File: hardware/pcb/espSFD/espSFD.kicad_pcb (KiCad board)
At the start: 2 copper layers, 68.6 x 34.3 mm, 9 parts, among them J1 Conn_01x06_Socket, J2 Conn_02x10_Odd_Even, Q1 IRLU3110Z, U1 WeMos_D1_mini, U2 TSR_1-2415

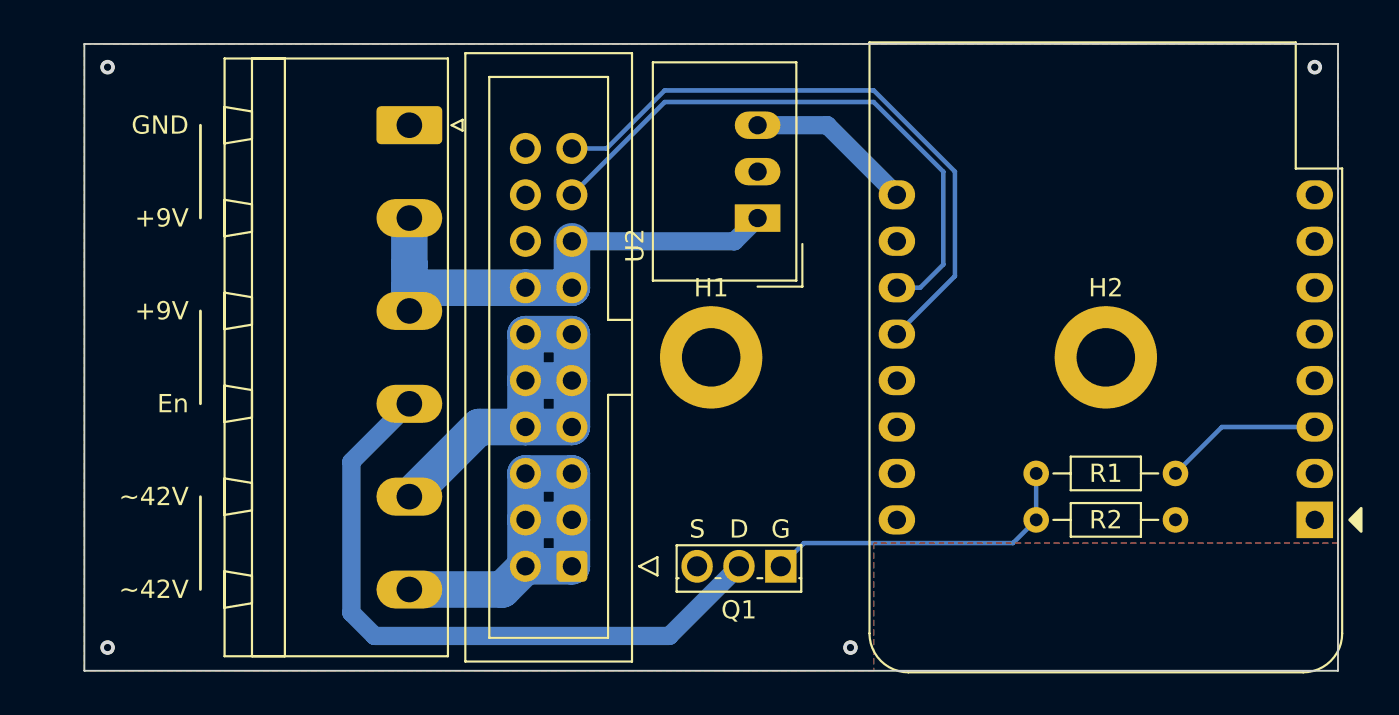
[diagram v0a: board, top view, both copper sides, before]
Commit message: es dghdgfj fcgj
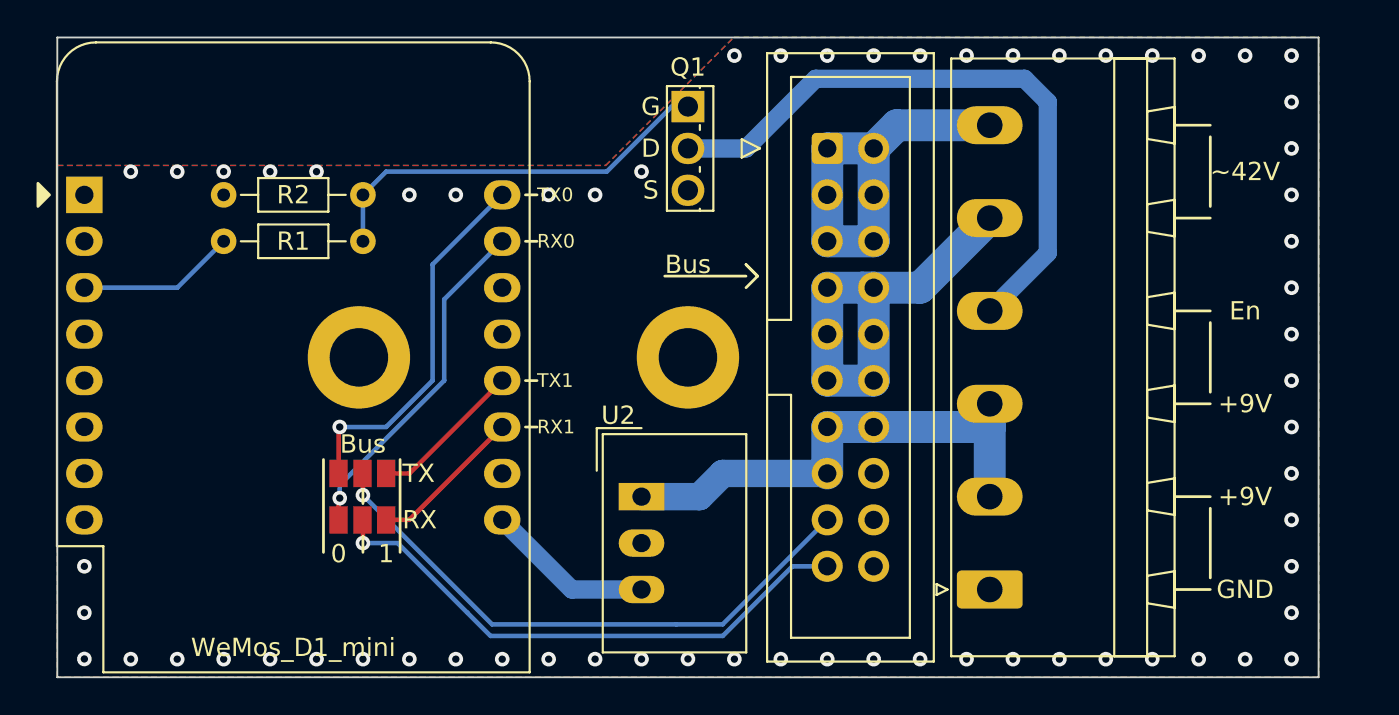
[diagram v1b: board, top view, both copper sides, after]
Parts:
- added JP1: SolderJumper_3_Open, Library:SolderJumper-3_P1.3mm_Open_Pad1.0x1.5mm no silk, F.Cu at (66.0, 102.9)
- added JP2: SolderJumper_3_Open, Library:SolderJumper-3_P1.3mm_Open_Pad1.0x1.5mm no silk, F.Cu at (66.0, 100.3)
- moved U1 69.6 mm to (50.8, 85.1), turned to 0 degrees
- moved R1 53.6 mm to (58.4, 87.6), turned to 0 degrees
- moved R2 40.9 mm to (66.0, 85.1), turned to 180 degrees
- moved H2 40.9 mm to (65.8, 94.0), turned to 180 degrees
- moved J1 40.7 mm to (100.3, 106.7), turned to 90 degrees
- moved J2 26.8 mm to (91.4, 82.5), turned to 0 degrees
- moved Q1 25.7 mm to (83.8, 80.3), turned to -90 degrees
- moved U2 16.5 mm to (81.3, 101.6), turned to -90 degrees
- moved H1 1.27 mm to (83.8, 94.0), turned to 180 degrees
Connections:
- J2 pad 17: RX -> TX
- J2 pad 19: TX -> RX
- U1 pad 11: RX -> RX1
- U1 pad 12: TX -> TX1
- U1 pad 15: unconnected-(U1-RX-Pad15) -> RX0
- U1 pad 16: unconnected-(U1-TX-Pad16) -> TX0
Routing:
- net TX0: track 0.00 -> 20.4 mm, vias 0 -> 1
- net RX0: track 0.00 -> 19.6 mm, vias 0 -> 1
- net TX1: track 0.00 -> 8.45 mm
- net RX1: track 0.00 -> 8.45 mm
- net Net-(Q1-G): track 17.6 -> 22.3 mm
- net Motor N: track 24.7 -> 22.1 mm
- net TX: track 34.3 -> 31.9 mm, vias 0 -> 1
- net Motor L: track 25.7 -> 23.8 mm
- net RX: track 32.1 -> 30.4 mm, vias 0 -> 1
- net En Motor: track 36.1 -> 34.5 mm
- net GND: vias 4 -> 64
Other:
- board size 68.6 x 34.3 mm -> 69 x 35 mm
- board text added: "0"
- board text added: "1"
- board text added: "Bus"
- board text added: "RX"
- board text added: "RX0"
- board text added: "RX1"
- board text added: "TX"
- board text added: "TX0"
- board text added: "TX1"
